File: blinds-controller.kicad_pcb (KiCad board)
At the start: 2 copper layers, 50.8 x 69.9 mm, 12 parts, among them J1 Jack-DC, J2 Stepper Motor, J3 DC Check, J4 JTAG, U1 MPM3610AGQV-P, U2 ESP32-S2-WROOM, U3 ULN2003A

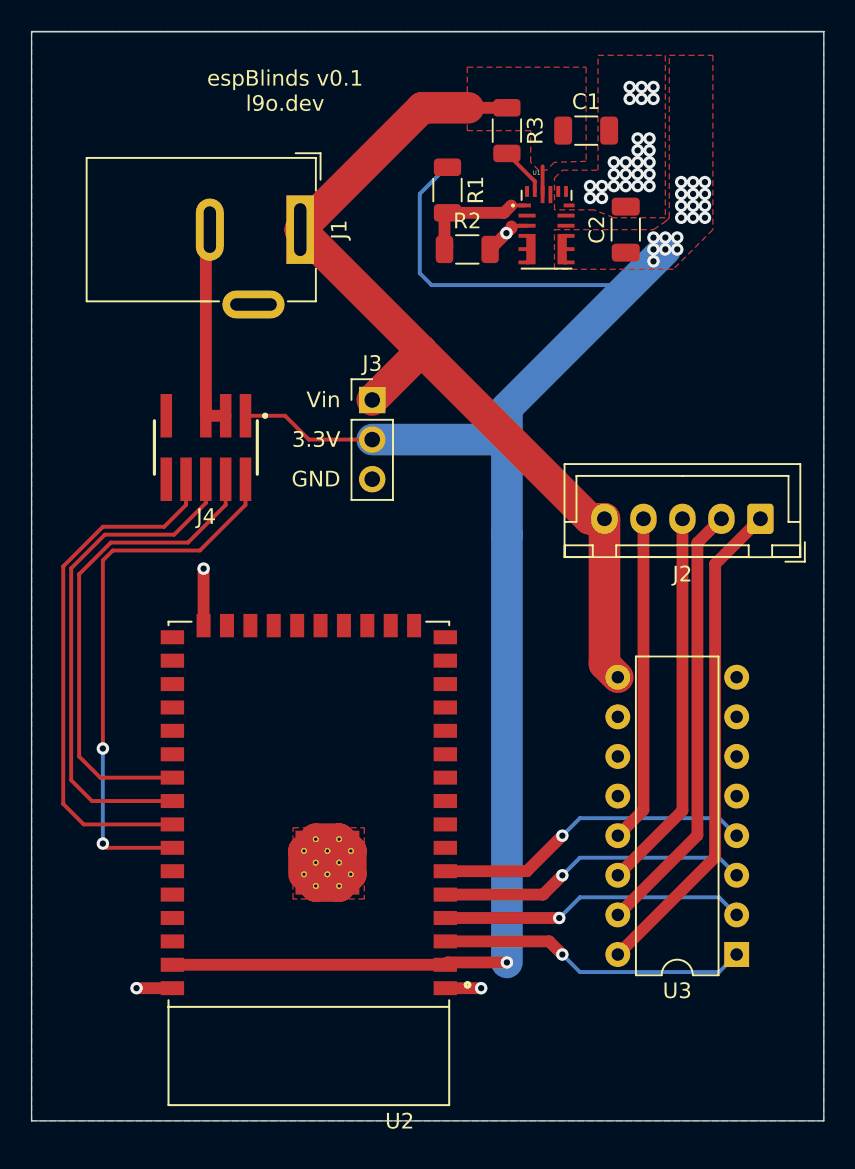
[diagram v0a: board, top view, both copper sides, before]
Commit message: Lots of small tweaks, almost there
Just missing decoupling capacitors and a final review
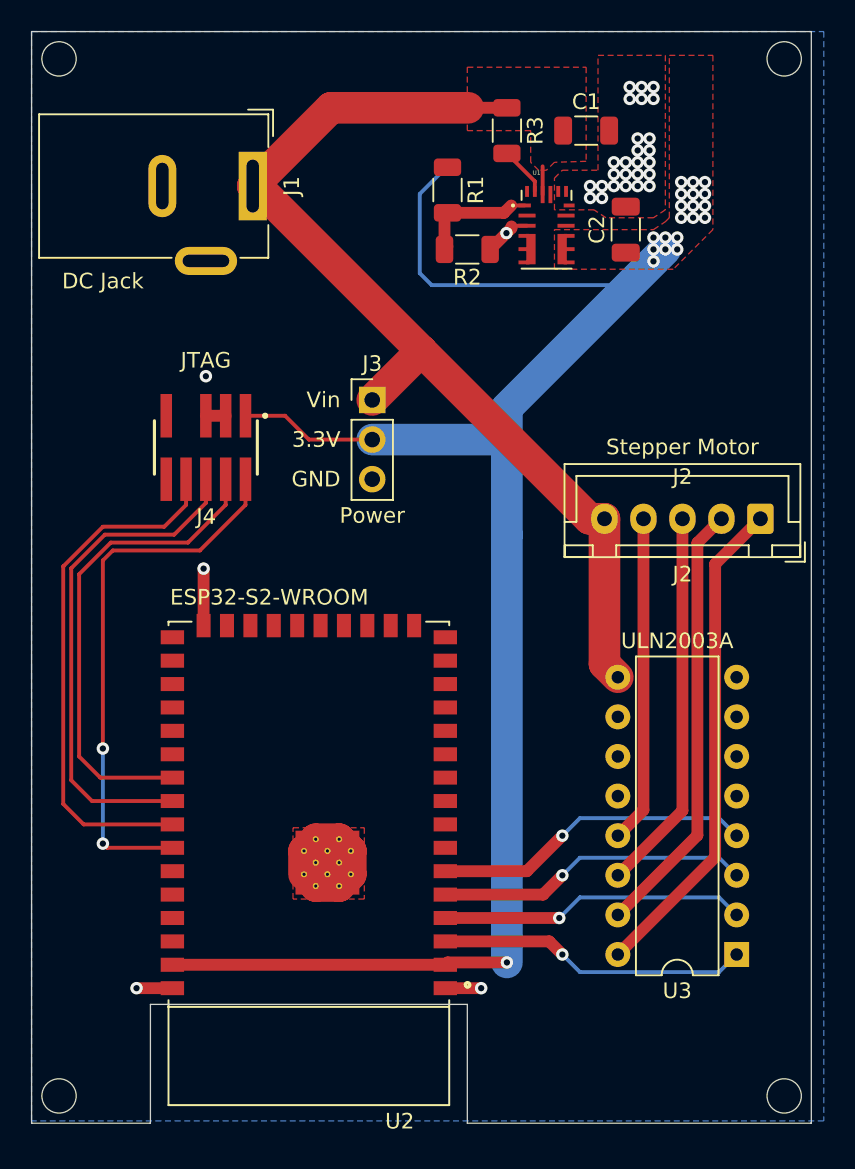
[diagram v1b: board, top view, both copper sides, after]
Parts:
- added REF**: MountingHole_2.2mm_M2_DIN965_Pad, MountingHole:MountingHole_2.2mm_M2_DIN965_Pad, F.Cu at (101.6, 20.8)
- added REF**: MountingHole_2.2mm_M2_DIN965_Pad, MountingHole:MountingHole_2.2mm_M2_DIN965_Pad, F.Cu at (101.6, 87.3)
- added REF**: MountingHole_2.2mm_M2_DIN965_Pad, MountingHole:MountingHole_2.2mm_M2_DIN965_Pad, F.Cu at (55.1, 87.3)
- added REF**: MountingHole_2.2mm_M2_DIN965_Pad, MountingHole:MountingHole_2.2mm_M2_DIN965_Pad, F.Cu at (55.1, 20.8)
- J1: value Jack-DC -> DC Jack
- J3: value DC Check -> Power
- moved J1 4.13 mm to (67.5, 29.0)
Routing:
- net GND: track 43.6 -> 31.5 mm, vias 30 -> 31
- net +12V: track 60.5 -> 66.6 mm
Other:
- board size 50.8 x 69.9 mm -> 50 x 70 mm
